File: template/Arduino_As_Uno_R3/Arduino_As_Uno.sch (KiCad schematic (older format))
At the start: 8 parts, among them P1 Power, P2 Analog, P3 Digital, P4 Digital, P5 CONN_1, P6 CONN_1, P7 CONN_1, P8 CONN_1

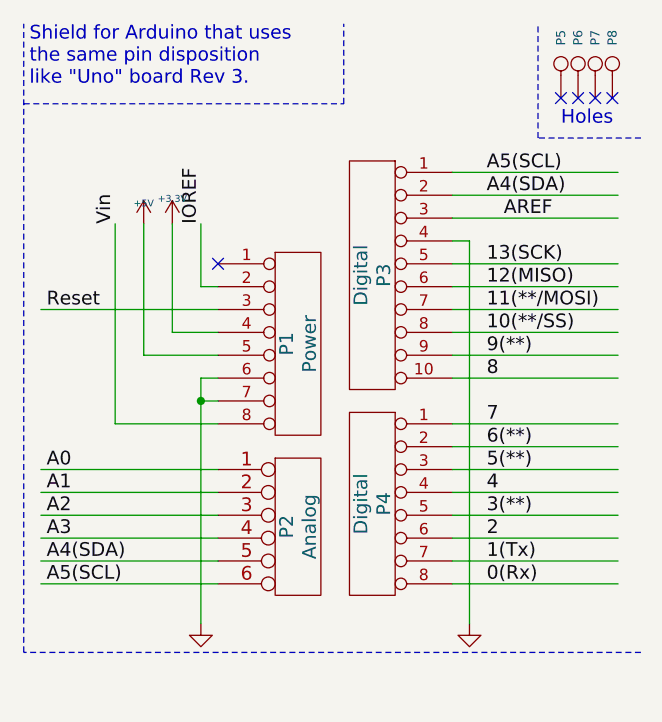
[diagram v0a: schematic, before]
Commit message: rebuilt shematic and fix librairie
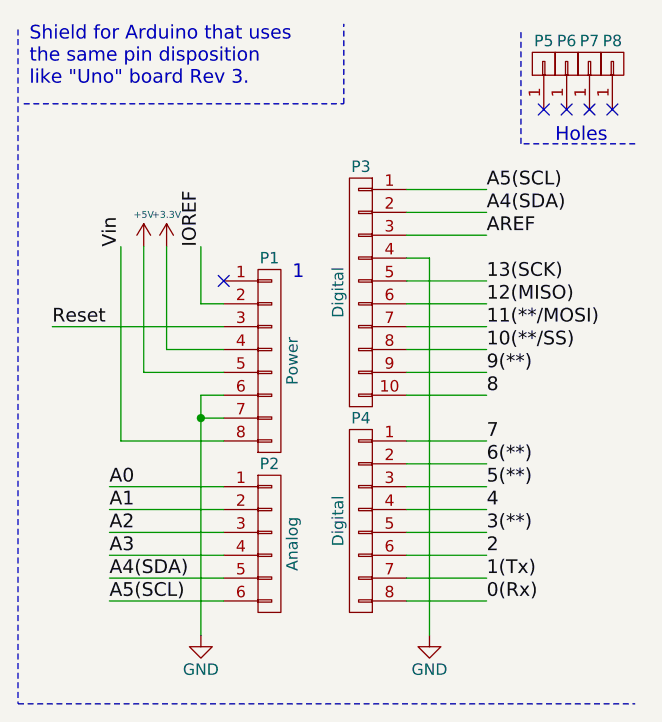
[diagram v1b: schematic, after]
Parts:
- removed P1: Power, Socket_Arduino_Uno:Socket_Strip_Arduino_1x08, symbol CONN_8
- removed P2: Analog, Socket_Arduino_Uno:Socket_Strip_Arduino_1x06, symbol CONN_6
- removed P3: Digital, Socket_Arduino_Uno:Socket_Strip_Arduino_1x10, symbol CONN_10
- removed P4: Digital, Socket_Arduino_Uno:Socket_Strip_Arduino_1x08, symbol CONN_8
- removed P5, P6, P7, P8: CONN_1, Socket_Arduino_Uno:Arduino_1pin, symbol CONN_1
- added P1: Power, Socket_Arduino_Uno:Socket_Strip_Arduino_1x08, symbol CONN_01X08
- added P2: Analog, Socket_Arduino_Uno:Socket_Strip_Arduino_1x06, symbol CONN_01X06
- added P3: Digital, Socket_Arduino_Uno:Socket_Strip_Arduino_1x10, symbol CONN_01X10
- added P4: Digital, Socket_Arduino_Uno:Socket_Strip_Arduino_1x08, symbol CONN_01X08
- added P5, P6, P7, P8: CONN_01X01, Socket_Arduino_Uno:Arduino_1pin, symbol CONN_01X01
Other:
- note added: "1"
